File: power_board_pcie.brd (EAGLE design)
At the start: 60 x 30 mm, 43 parts, among them J1 PCIE_EDGE, U1 74HCT08D

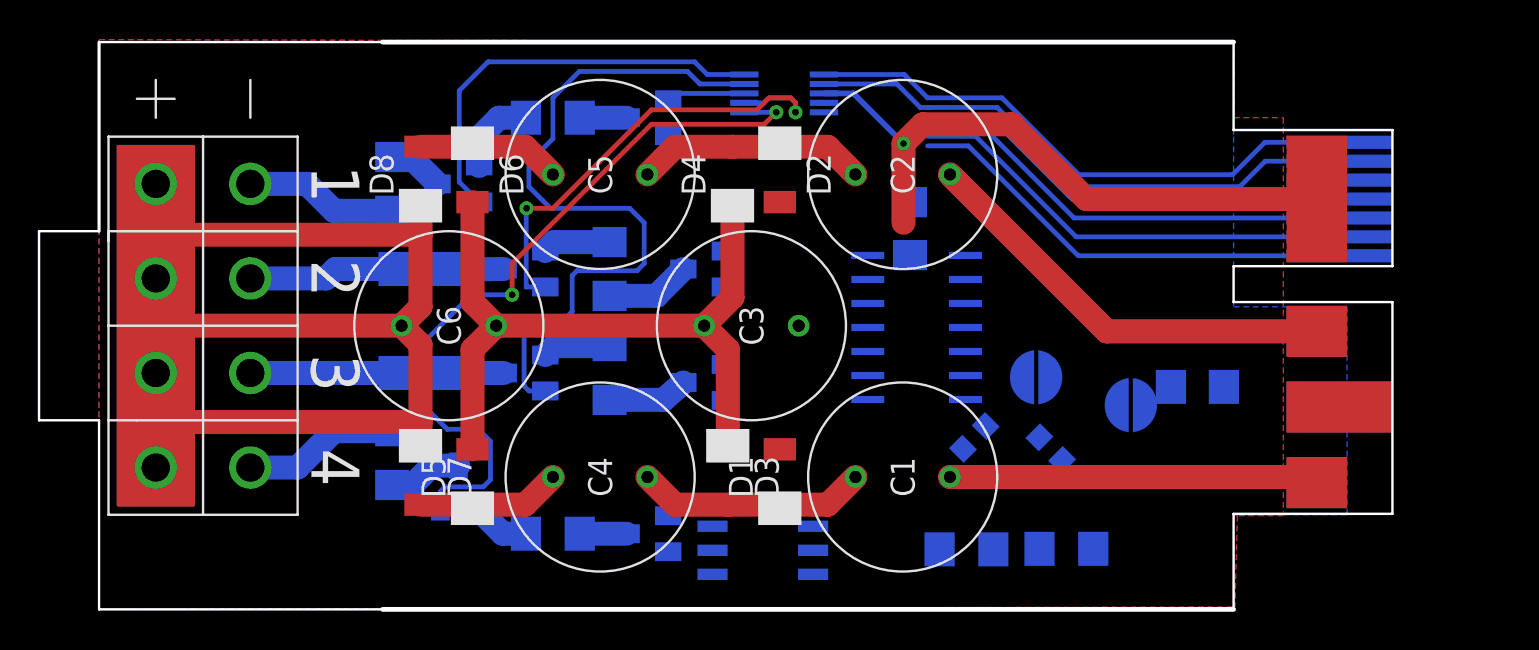
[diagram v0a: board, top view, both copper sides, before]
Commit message: Update 9-26
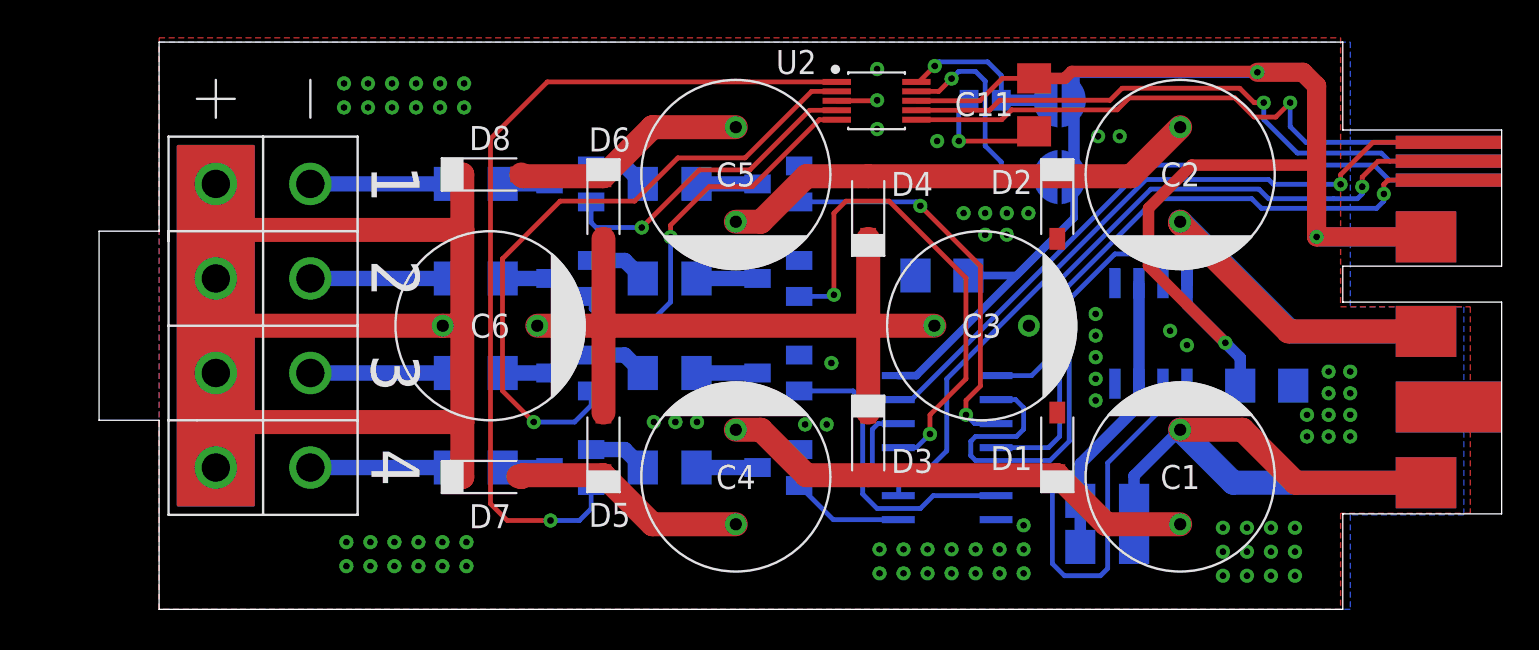
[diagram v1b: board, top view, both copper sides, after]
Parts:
- removed U$1: AZ4558CMTR-G1, tide_clock:SOIC127P600X175-8
- removed U$2: DAC5574, tide_clock:SOP50P490X110-10
- added C7: (no value), resistor:C1206
- added U2: DAC5574, tide_clock:SOP50P490X110-10
- added U3: AZ4558CMTR-G1, tide_clock:SOIC127P600X175-8
- D1, D2, D3, D4, D5, D6, D7, D8: value CD1206-S01575 -> BAS16GW; device tide_clock:DIOC3215X95 -> tide_clock:SOD3616X130
- moved R12 18.7 mm to (46.9, 26.9), turned to 0 degrees
- moved JP2 16.6 mm to (50.8, 26.9)
- moved D1 14.8 mm to (50.7, 8.75)
- moved D2 14.8 mm to (50.7, 21.2)
- moved C1 14.7 mm to (57.2, 7.00), turned to 180 degrees
- moved C2 14.7 mm to (57.2, 23.0), turned to 0 degrees
- moved R11 13.8 mm to (46.9, 22.9), turned to 0 degrees
- moved C3 12.2 mm to (46.7, 15.0)
- moved JP1 10.7 mm to (50.8, 22.9), turned to 0 degrees
- moved C11 9.27 mm to (49.5, 26.7), flipped to the top
- moved T5 7.76 mm to (35.9, 7.50)
- moved T8 7.76 mm to (35.9, 22.5)
- moved D3 7.63 mm to (40.7, 8.75)
- moved R2 7.44 mm to (53.3, 3.30), turned to 0 degrees
- moved D4 7.39 mm to (40.7, 21.2)
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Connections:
- net +5V: now also C7.1, J1.PWR3_2, JP1.1, JP2.1, U2.8, U3.8; no longer R11.2, R12.2, U$1.8, U$2.8
- net EN1: now also J1.P6; no longer J1.P$17
- net EN2: now also J1.P3; no longer J1.P$16
- net EN3: now also J1.P2; no longer J1.P$15
- net EN4: now also J1.P1; no longer J1.P$14
- net GND: now also C7.2, R11.2, R12.2, U2.3, U3.2, U3.4, U3.5; no longer JP1.1, JP2.1, U$1.2, U$1.4, U$1.5, U$2.3
- net N$2: now also U3.3, U3.6; no longer U$1.3, U$1.6
- net N$20: now also U2.2; no longer U$2.4
- net N$21: now also U2.5; no longer U$2.2
- net N$22: now also U2.4; no longer U$2.5
- net N$23: now also U2.1; no longer U$2.1
- net N$32: now also U2.9; no longer U$2.9
- net N$33: now also U2.10; no longer U$2.10
- net PH_EN1: now also U1.12, U1.9, U3.1; no longer U$1.1, U1.2, U1.5
- net PH_EN2: now also U1.2, U1.5, U3.7; no longer U$1.7, U1.12, U1.9
- net SCL: now also J1.P4, U2.6; no longer J1.P$20, U$2.6
- net SDA: now also J1.P5, U2.7; no longer J1.P$19, U$2.7
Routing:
- net +5V: track 33.4 -> 104.4 mm, vias 1 -> 3
- net PH_EN1: track 0.00 -> 33.9 mm
- net PH_EN2: track 0.00 -> 27.7 mm
- net SW4: track 0.00 -> 26.1 mm, vias 0 -> 2
- net SW1: track 0.00 -> 21.0 mm, vias 0 -> 2
- net SW2: track 0.00 -> 16.2 mm
- net EN2: track 23.8 -> 39.1 mm, vias 0 -> 1
- net N$2: track 0.00 -> 15.2 mm
- net PWR2: track 45.7 -> 30.9 mm
- net N$6: track 12.2 -> 25.6 mm
- net N$5: track 12.2 -> 25.6 mm
- net N$32: track 0.00 -> 11.5 mm, vias 0 -> 1
- net EN1: track 23.6 -> 34.6 mm
- net EN4: track 24.2 -> 35.1 mm, vias 0 -> 1
- net N$33: track 0.00 -> 8.35 mm, vias 0 -> 1
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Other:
- board size 60 x 30 mm -> 74.2 x 30 mm
- board text added: "A0"
- board text added: "A1"
